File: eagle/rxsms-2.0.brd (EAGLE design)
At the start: 159 x 120.5 mm, 164 parts, among them Q1 opt, Q10 BSS123, Q11 BSS123, Q12 BSS123, Q2 BSS123, Q3 BSS123, Q4 BSS123, Q5 BSS123, Q6 BSS123, Q7 BSS123, Q8 BSS123, Q9 BSS123, T10_SODS SWITCH_LED, T1_LO SMS_IP67, T2_SOE SMS_IP67, T3_SOE SWITCH_LED, T4_PWR SMS_IP67, T5_ERRINH SMS_IP67, T6_PWR SWITCH_LED, T7_ERRINH SWITCH_LED, T8_LO SWITCH_LED, T9_SODS SMS_IP67, U1 MAX3232ESE, U2 XMEGA-A4UTQFP, U3 TSR_1-2450, U4 LM1117, U5 NC7WZ17P6X, U6 ADUM3160, U7 TPS73125, U8 NUP2202W1, X1 PN61729-S, X5 RLP2-200-500

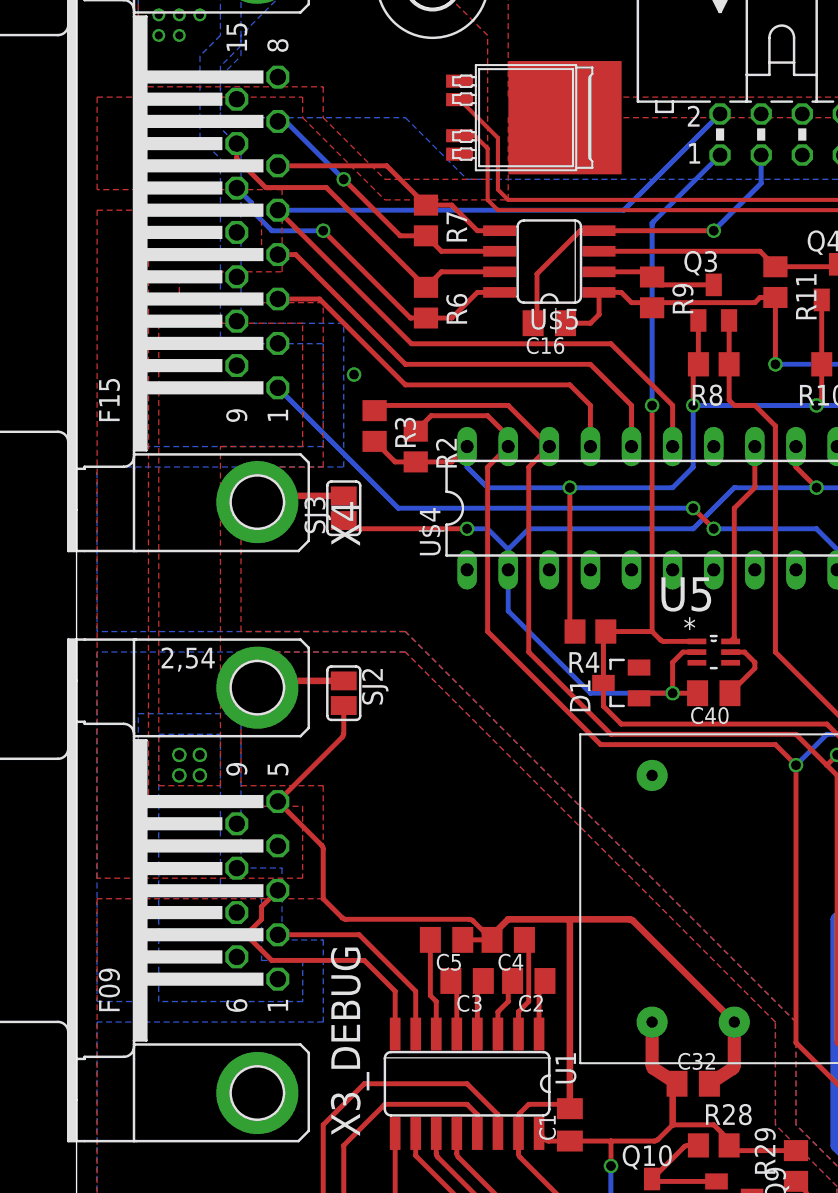
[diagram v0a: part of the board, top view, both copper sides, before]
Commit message: added even more OC
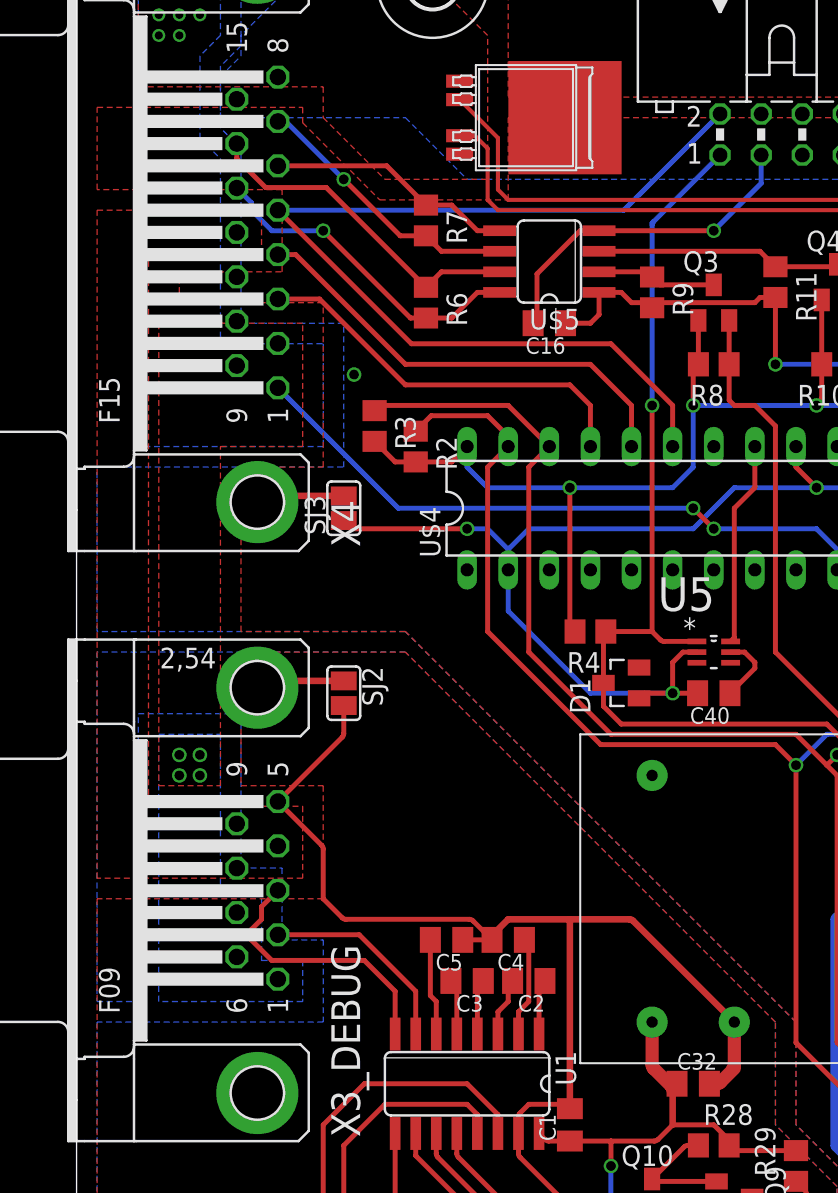
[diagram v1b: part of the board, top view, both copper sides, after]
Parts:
- C17, C18, C19, C20: value >100n/low ESR -> 1u
- R29, R32: value 267 -> 270
- R43, R44: value 220 -> 68
- R49: value 220 -> 150
- U$7_BER, U$8_DROPR, U$9_DROPDUR: value (none) -> 50k
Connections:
- net GND: now also U5.3
